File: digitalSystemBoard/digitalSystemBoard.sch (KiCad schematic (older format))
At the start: 14 parts, among them J1 Barrel_Jack, Q1 MJD122T4G, SW1 SW_SPDT, U1 LM317

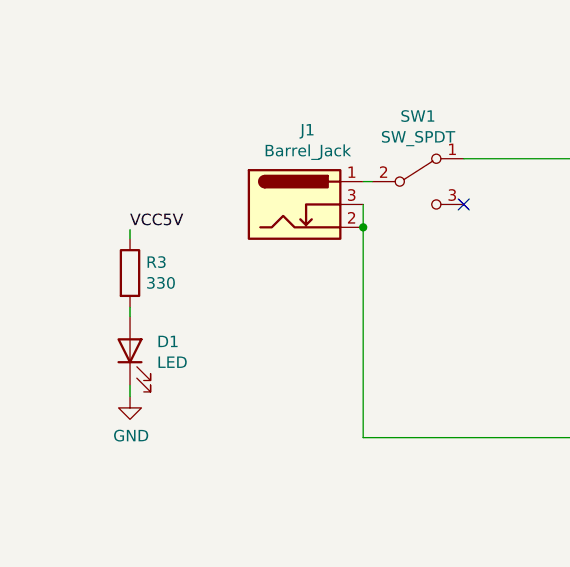
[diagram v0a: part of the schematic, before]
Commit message: Debug error part 2
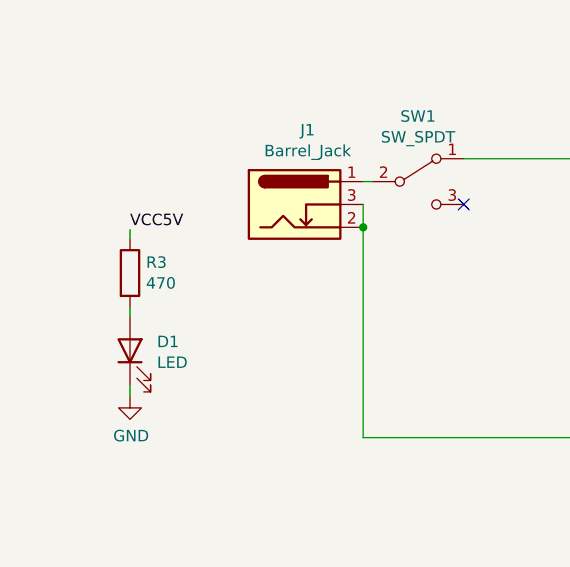
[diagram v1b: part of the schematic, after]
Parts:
- R3: value 330 -> 470
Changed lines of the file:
@@
-$EndComp
-$Comp
-L Device:R R3
-U 1 1 5FB7DD09
-P 980 1970
-F 0 "R3" H 1050 2016 50  0000 L CNN
-F 1 "330" H 1050 1925 50  0000 L CNN
-F 2 "Resistor_SMD:R_0603_1608Metric" V 910 1970 50  0001 C CNN
-F 3 "~" H 980 1970 50  0001 C CNN
-	1    980  1970
-	1    0    0    -1
 $EndComp
 $Comp
@@
 	4470 2350 4260 2350
 Connection ~ 4470 2000
+$Comp
+L Device:R R3
+U 1 1 5FB7DD09
+P 980 1970
+F 0 "R3" H 1050 2016 50  0000 L CNN
+F 1 "470" H 1050 1925 50  0000 L CNN
+F 2 "Resistor_SMD:R_0603_1608Metric" V 910 1970 50  0001 C CNN
+F 3 "~" H 980 1970 50  0001 C CNN
+	1    980  1970
+	1    0    0    -1
+$EndComp
 $EndSCHEMATC
